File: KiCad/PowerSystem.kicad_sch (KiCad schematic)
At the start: 21 parts, among them J14 powerRailAndBatteryGround, J15 Barrel_Jack_Switch, J16 Barrel3andbarrel2, J18 positivePowerInputs, SW8 SW_DIP_x01, U1 LT1054, U13 MCP1703T-5002E/DB, U14 MCP1703T-5002E/DB, U15 MCP1703T-3302E/DB, U2 PMEG2005CT_215

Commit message: Changes to the BoM
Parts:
- C24: Part_Number (none) -> UWT1H100MCL1GB
- C25: Part_Number (none) -> 865080545012
- C26, C27: Part_Number (none) -> 865060640001
- C28, C29, C30, C31, C33, C34: Part_Number (none) -> C0603C105K4RACTU
- J14, J16: Part_Number (none) -> SSK02-FPH-254-A2
- J18: Part_Number (none) -> SSK02-FPH-254-A3
- U1: Part_Number (none) -> LT1054CDWR
- U13, U14: Part_Number (none) -> MCP1703-5002E/DB
- U15: Part_Number (none) -> MCP1703-3302E/DB
- U2: Part_Number (none) -> PMEG2005CT,215

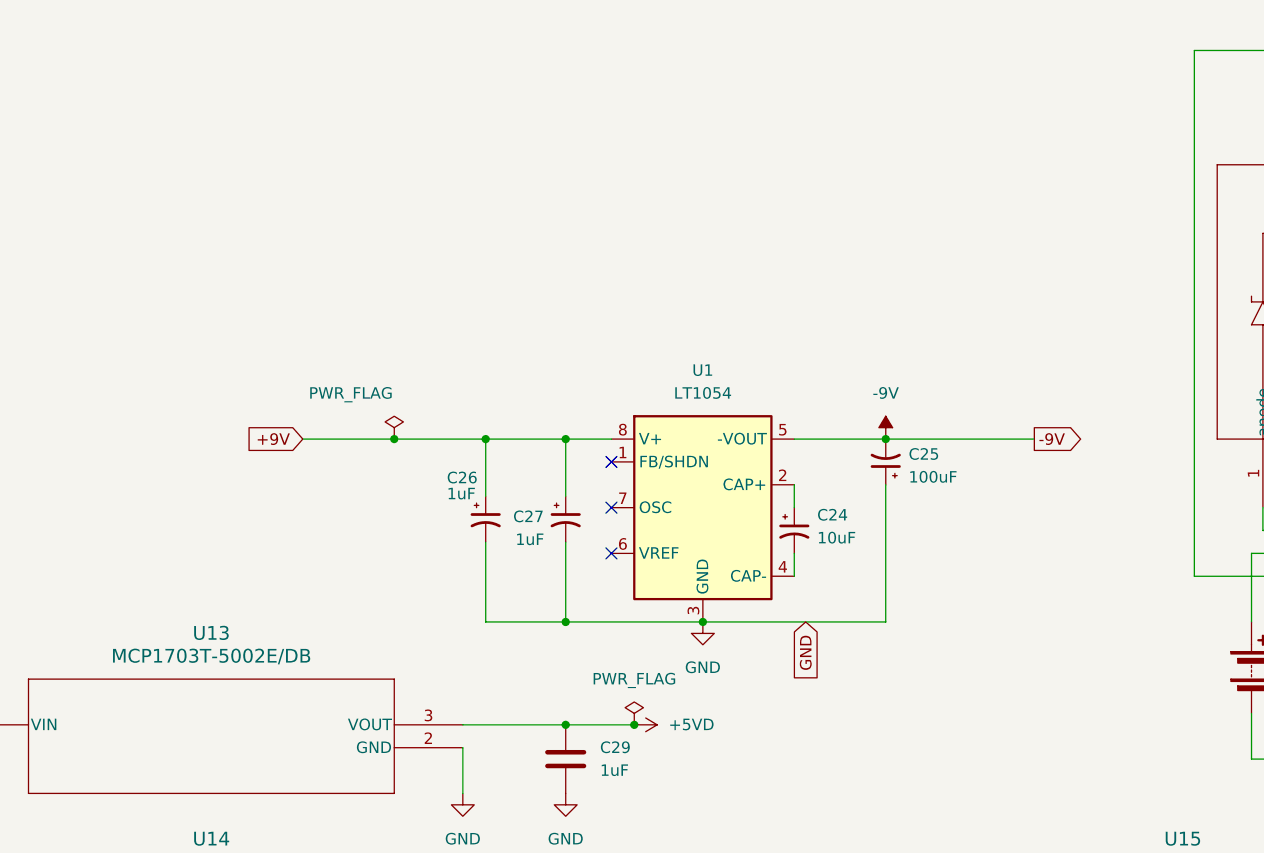
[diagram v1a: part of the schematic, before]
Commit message: done
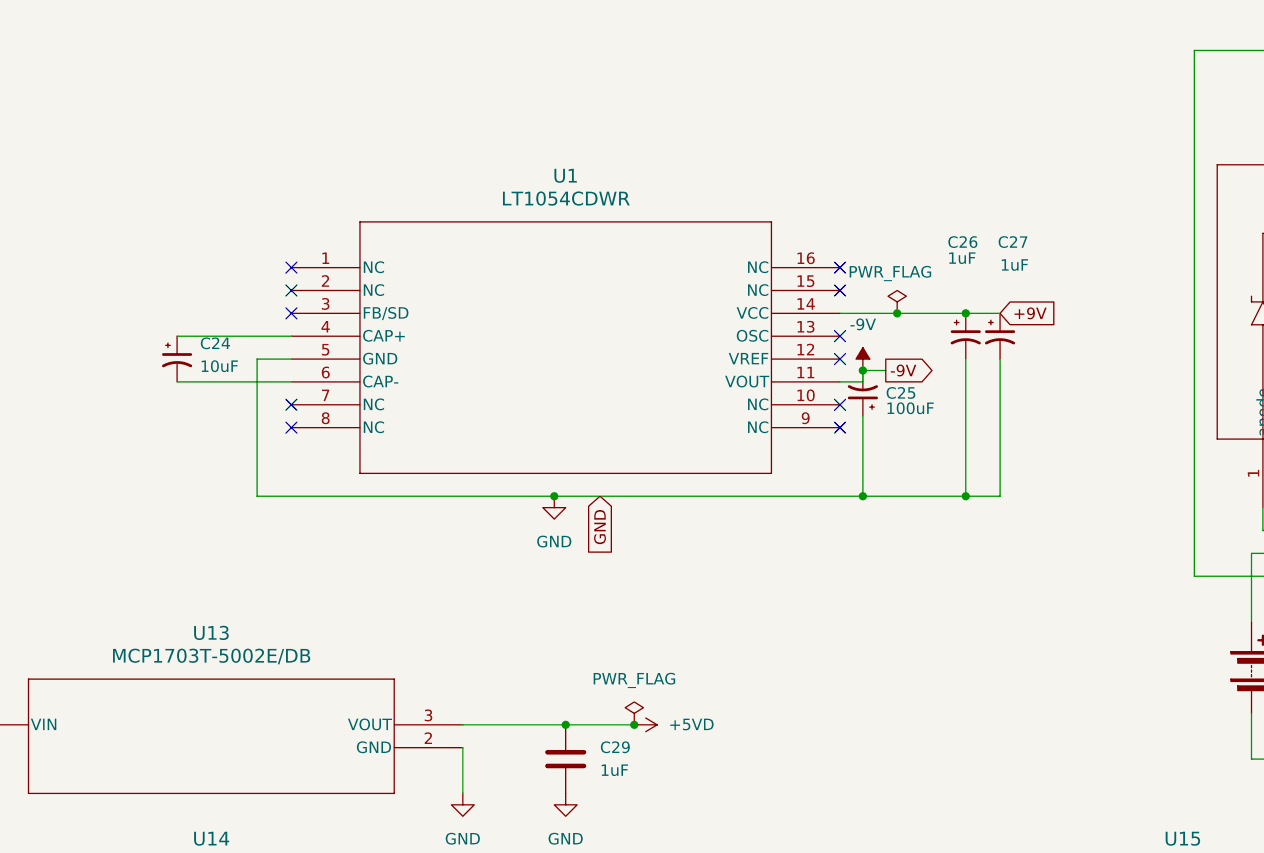
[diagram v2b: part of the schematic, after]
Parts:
- removed U1: LT1054, charge_pump:SOIC127P1030X265-16N, symbol Regulator_SwitchedCapacitor:LT1054
- added U1: LT1054CDWR, lt1054_16soic:DW16-M, symbol lt1054_soic16:LT1054CDWR
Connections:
- net +9V: now also U1.14 (VCC)
- net -9V: now also U1.11 (VOUT)
- net GND: now also U1.5 (GND)
- net at C24.1: now also U1.4 (CAP+)
- net at C24.2: now also U1.6 (CAP-)
- no-connect marks 3 -> 11
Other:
- moved on the sheet: C24, C25, C26, C27
